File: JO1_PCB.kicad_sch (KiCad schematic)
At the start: 25 parts, among them J1 CN8, J10 ESC_PWM, J11 CAN_WCMCU-1051_BLUEPILL, J12 TFT, J13 LM2596_3.3V, J14 LM2596_5V, J2 CN7, J3 CN9, J4 CN10, J5 MPU-6050, J6 CAN_WCMCU-1051_NUCLEO, J7 SERVO, J8 DC_MOTOR, J9 ESC_MOTOR, SW1 SW_Nidec_CAS-120A1, U1 NRF24L01, U2 BP

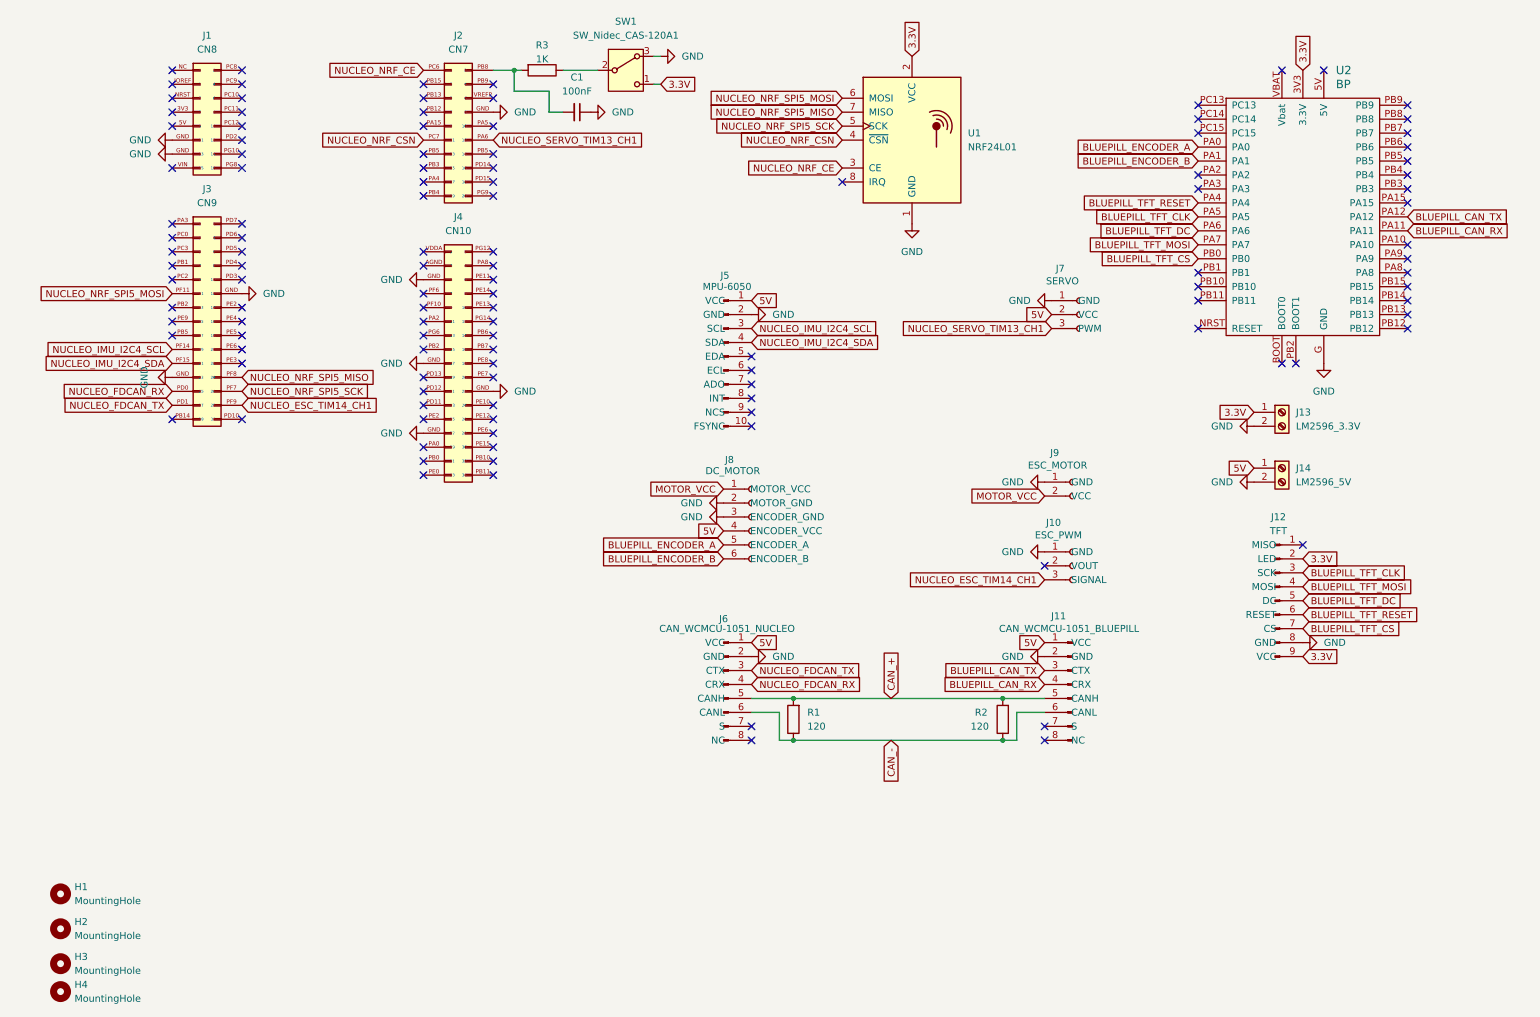
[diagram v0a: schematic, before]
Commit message: Version Nov 21
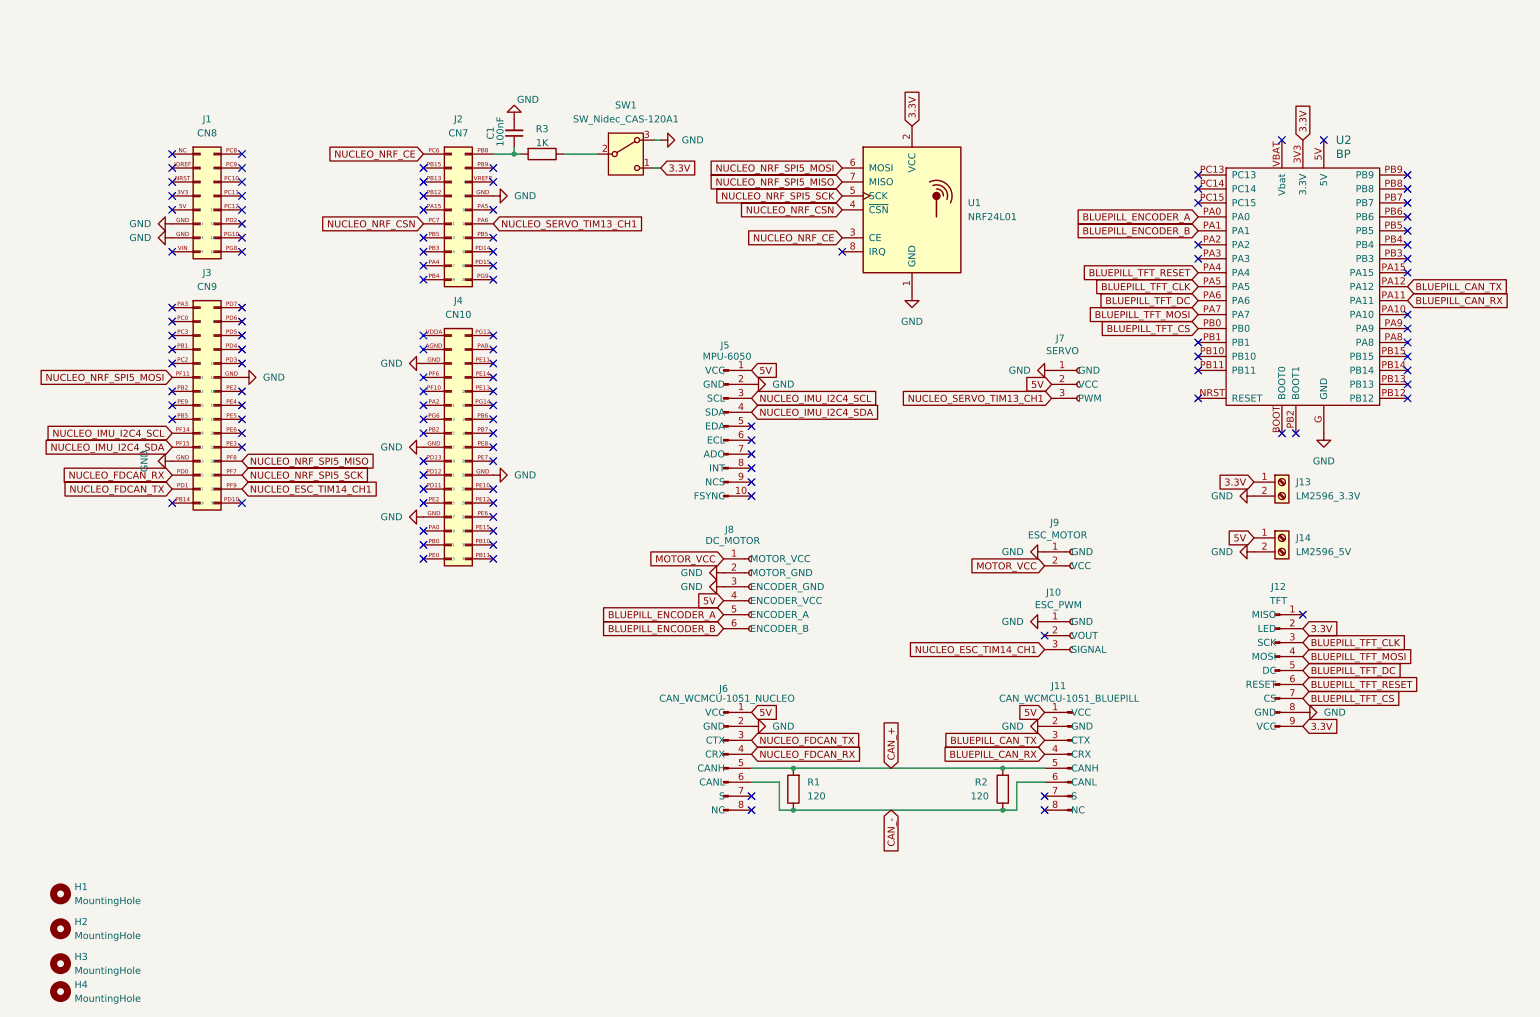
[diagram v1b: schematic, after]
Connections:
- net GND: now also C1.2; no longer C1.1
- net at J2.PB8 (2), R3.2: now also C1.1; no longer C1.2
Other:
- moved on the sheet: C1, J1, J10, J11, J12, J13, J14, J2, J3, J4, J5, J6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
